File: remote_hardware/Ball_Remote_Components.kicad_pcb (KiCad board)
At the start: 4 copper layers, 92.3 x 128.5 mm, 77 parts, among them J1 Eurorack_10_pin_power, J2 SWD_Header, J3 USB_B_Micro, J4 X_Out, J5 Y_Out, J6 Z_Out, U1 STM32WB35, U2 LD1117-3.3-4Tab, U3 TL074, U4 TL072, Y1 32MHz

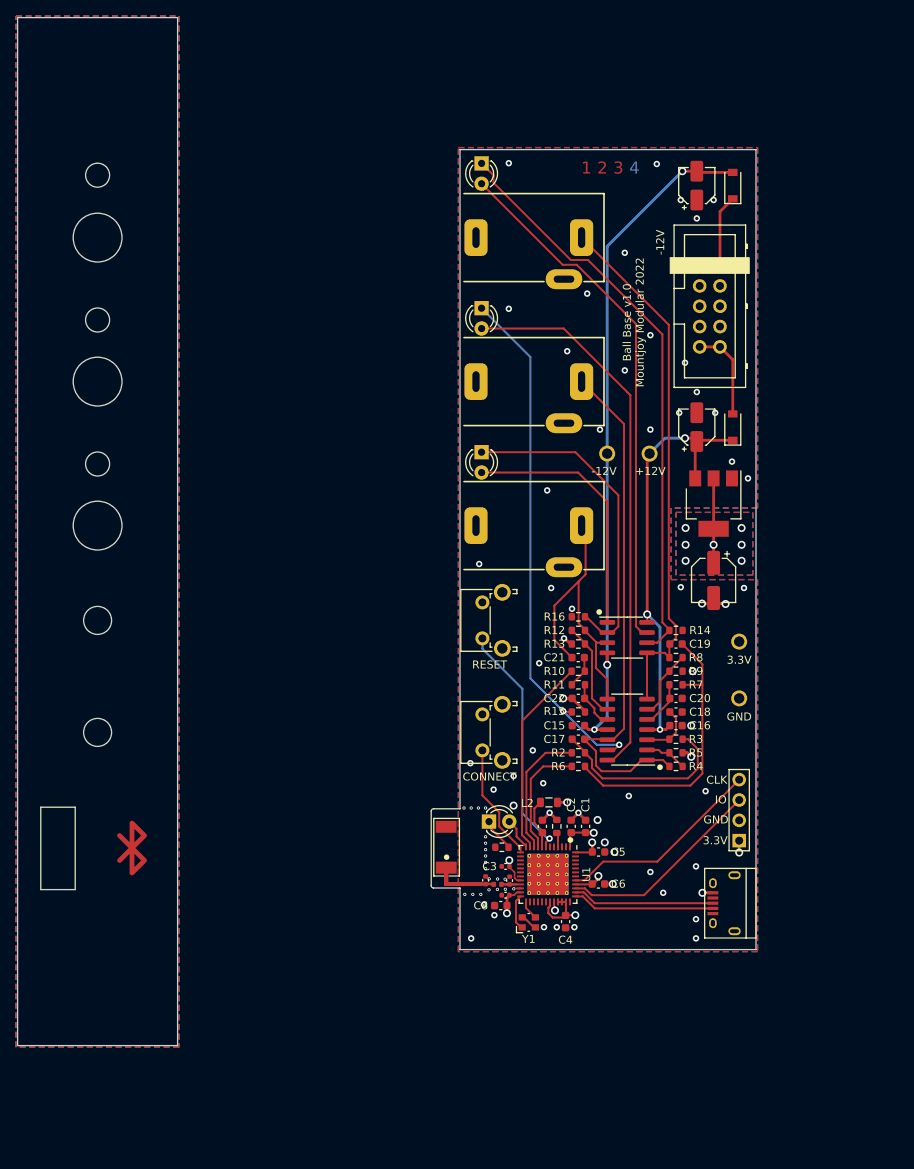
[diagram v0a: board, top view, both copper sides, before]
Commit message: Work on remote PCB
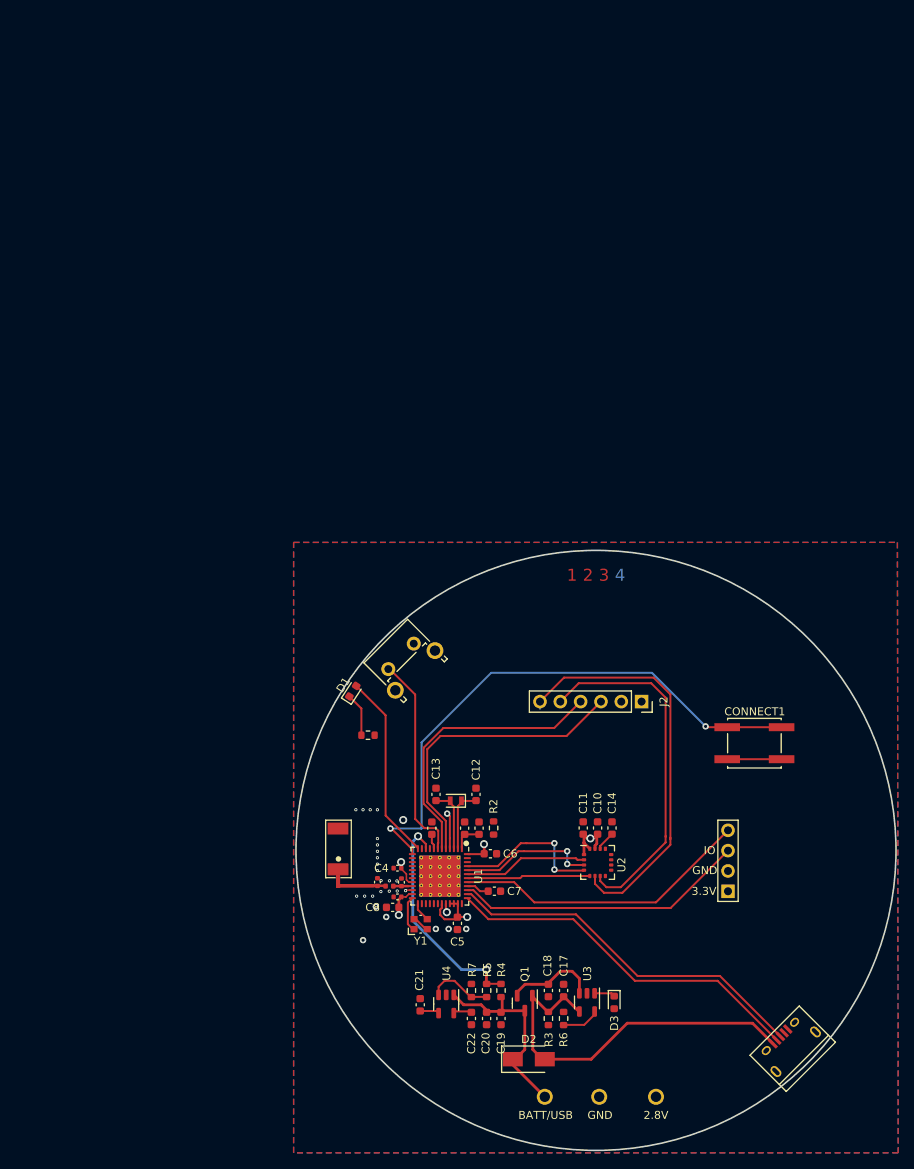
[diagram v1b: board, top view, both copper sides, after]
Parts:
- removed the C15 at (140.4, 128.0)
- removed the C16 at (152.6, 128.0)
- removed the D1 at (159.7, 90.7)
- removed D4: LED_X, LED_THT:LED_D3.0mm_FlatTop
- removed D5: LED_Y, LED_THT:LED_D3.0mm_FlatTop
- removed D6: LED_Z, LED_THT:LED_D3.0mm_FlatTop
- removed G***: LOGO, Custom_Footprints:bluetooth
- removed the J1 at (155.6, 70.5)
- removed J4: X_Out, Custom_Footprints:Jack_3.5mm_QingPu_WQP-PJ302M_Horizontal
- removed J5: Y_Out, Custom_Footprints:Jack_3.5mm_QingPu_WQP-PJ302M_Horizontal
- removed J6: Z_Out, Custom_Footprints:Jack_3.5mm_QingPu_WQP-PJ302M_Horizontal
- removed L2: L, Inductor_SMD:L_0805_2012Metric
- removed R10, R11: 20k, Resistor_SMD:R_0603_1608Metric
- removed R12, R8: 5k1, Resistor_SMD:R_0603_1608Metric
- removed R13, R9: 10k, Resistor_SMD:R_0603_1608Metric
- removed R14, R15, R16: 1k, Resistor_SMD:R_0603_1608Metric
- removed the R2 at (140.4, 131.4)
- removed Ref** (x3): Thonkikonn_6.1mm, Custom_Footprints:MountingHole_6.1mm
- removed Ref** (x3): LED_Hole_3mm, Custom_Footprints:LED_Hole_3mm
- removed Ref** (x2): Oval_Mounting_Hole, Custom_Footprints:Oval_Mounting_Hole
- removed Ref** (x2): Push_Button_Hole, Custom_Footprints:Small_Pushbutton_Hole_3.5mm
- removed TP4: TestPoint, Custom_Footprints:1.3mm_Test_Point
- added C12: 16pF, Capacitor_SMD:C_0603_1608Metric, F.Cu at (127.6, 136.6)
- added C13: 16pF, Capacitor_SMD:C_0603_1608Metric, F.Cu at (122.6, 136.6)
- added D3: LED_CHG, LED_SMD:LED_0603_1608Metric, F.Cu at (144.9, 162.6)
- added J2: I2C_Gyro_Module, Connector_PinSocket_2.54mm:PinSocket_1x06_P2.54mm_Vertical, F.Cu at (148.3, 125.0)
- added Q1: SI2333DS, Package_TO_SOT_SMD:SOT-23, F.Cu at (133.7, 162.7)
- added Y2: 32.768MHz, Crystal:Crystal_SMD_2012-2Pin_2.0x1.2mm, F.Cu at (125.1, 137.4)
- C10: value 22uF -> 100nF; footprint Capacitor_SMD:CP_Elec_4x5.4 -> Capacitor_SMD:C_0603_1608Metric
- C11: value 22uF -> 10uF; footprint Capacitor_SMD:CP_Elec_4x5.4 -> Capacitor_SMD:C_0603_1608Metric
- C14: value 47uF -> 10nF; footprint Capacitor_SMD:CP_Elec_5x5.8 -> Capacitor_SMD:C_0603_1608Metric
- C17: value 22nF -> 4.7uF
- C18: value 33nF -> 4.7uF
- C19: value 22nF -> 1uF
- C20, C22: value 33nF -> 1uF
- C21: value 22nF -> 10nF
- CONNECT1: footprint Button_Switch_THT:SW_Tactile_SPST_Angled_PTS645Vx58-2LFS -> Button_Switch_SMD:SW_SPST_EVQQ2
- D1: renamed from D3; value LED_BLUE -> LED_CONNECT; footprint LED_THT:LED_D3.0mm_FlatTop -> LED_SMD:LED_0603_1608Metric
- D2: value 1N5819 -> PMEG3010ER; footprint Diode_SMD:D_SOD-123 -> Diode_SMD:D_SMA
- R3: value 20k -> 1k
- R4: value 5k1 -> 27k
- R5: value 10k -> 13k
- R6: value 20k -> 10k
- R7: value 20k -> 24k
- U2: value LD1117-3.3-4Tab -> L3GD20; footprint Package_TO_SOT_SMD:SOT-223-3_TabPin2 -> Package_LGA:LGA-16_4x4mm_P0.65mm_LayoutBorder4x4y
- U3: value TL074 -> MCP73831-2-OT; footprint Package_SO:SOIC-14_3.9x8.7mm_P1.27mm -> Package_TO_SOT_SMD:SOT-23-5
- U4: value TL072 -> LD3985M28R_SOT23; footprint Package_SO:SOIC-8_3.9x4.9mm_P1.27mm -> Package_TO_SOT_SMD:SOT-23-5
- moved D2 112.1 mm to (134.2, 169.7), turned to 0 degrees
- moved C11 81.5 mm to (141.0, 140.8)
- moved TP3 81.5 mm to (136.2, 174.4), turned to -90 degrees
- moved TP2 57.8 mm to (150.1, 174.4), turned to 0 degrees
- moved TP1 52.8 mm to (143.0, 174.4), turned to 0 degrees
- moved C19 51.7 mm to (130.7, 164.6), turned to -90 degrees
- moved C10 51.6 mm to (142.8, 140.8)
- moved U4 51.1 mm to (123.9, 162.8), turned to -90 degrees
- moved FID1 50.9 mm to (142.6, 109.2)
- moved C21 47.7 mm to (120.6, 162.9), turned to 90 degrees
- moved U2 47.1 mm to (142.8, 145.1), turned to 0 degrees
- moved C20 46.5 mm to (128.9, 164.6), turned to -90 degrees
- moved R7 46.0 mm to (127.0, 161.1), turned to 90 degrees
- moved C22 42.2 mm to (127.0, 164.6), turned to -90 degrees
- moved R3 38.4 mm to (136.7, 164.6), turned to 90 degrees
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- renumbered C7 to C1, C12 to C15, C13 to C16, C1 to C2, C2 to C3, C3 to C4, C4 to C5, C5 to C6, C6 to C7, J3 to J1, J2 to J3, R17 to R1, R1 to R2
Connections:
- C1 pad 2: +3.3VA -> +2V8
- C10 pad 1: VCC -> +2V8
- C11 pad 1: GND -> +2V8
- C11 pad 2: VEE -> GND
- C14 pad 1: +3V3 -> Net-(C14-Pad1)
- C17 pad 1: /Y_Filtered -> /USB_VIN
- C17 pad 2: Net-(C17-Pad2) -> GND
- C18 pad 1: GND -> /BATT_+
- C18 pad 2: Net-(C18-Pad2) -> GND
- C19 pad 1: /X_Filtered -> VCC
- C19 pad 2: Net-(C19-Pad2) -> GND
- C2 pad 1: +3V3 -> +2V8
- C20 pad 1: GND -> VCC
- C20 pad 2: Net-(C20-Pad2) -> GND
- C21 pad 1: /Z_Filtered -> Net-(C21-Pad1)
- C21 pad 2: Net-(C21-Pad2) -> GND
- C22 pad 1: GND -> +2V8
- C22 pad 2: Net-(C22-Pad2) -> GND
- C3 pad 1: +3V3 -> +2V8
- C4 pad 1: +3V3 -> +2V8
- C5 pad 1: +3V3 -> +2V8
- C6 pad 1: +3V3 -> +2V8
- C7 pad 1: +3V3 -> +2V8
- C8 pad 1: +3V3 -> +2V8
- C9 pad 1: +3V3 -> +2V8
- D2 pad 1: -12V -> VCC
- D2 pad 2: VEE -> /USB_VIN
- J1 pad 1: unconnected-(J3-Pad1) -> /USB_VIN
- R3 pad 1: Net-(C17-Pad2) -> Net-(D3-Pad2)
- R3 pad 2: Net-(C18-Pad2) -> /USB_VIN
- R4 pad 1: Net-(R4-Pad1) -> VCC
- R4 pad 2: /Y_Filtered -> /Battery_Level
- R5 pad 1: GND -> /Battery_Level
- R5 pad 2: Net-(R4-Pad1) -> /LDO_Inhibit
- R6 pad 1: /X_PWM -> GND
- R6 pad 2: Net-(C19-Pad2) -> Net-(R6-Pad2)
- R7 pad 1: Net-(C19-Pad2) -> /LDO_Inhibit
- R7 pad 2: Net-(C20-Pad2) -> GND
- TP2 pad 1: +3V3 -> +2V8
- U1 pad 1: +3V3 -> +2V8
- U1 pad 10: /Y_PWM -> /Battery_Level
- U1 pad 11: /Z_PWM -> unconnected-(U1-Pad11)
- U1 pad 2: unconnected-(U1-Pad2) -> Net-(C12-Pad2)
- U1 pad 20: +3V3 -> +2V8
- U1 pad 23: +3V3 -> +2V8
- U1 pad 3: unconnected-(U1-Pad3) -> Net-(C13-Pad2)
- U1 pad 31: +3V3 -> +2V8
- U1 pad 33: +3V3 -> +2V8
- U1 pad 34: +3V3 -> +2V8
- U1 pad 35: +3V3 -> +2V8
- U1 pad 36: unconnected-(U1-Pad36) -> /LDO_Inhibit
- U1 pad 40: +3V3 -> +2V8
- U1 pad 42: unconnected-(U1-Pad42) -> /SPI_CS
- U1 pad 43: unconnected-(U1-Pad43) -> /SPI_CLK
- U1 pad 44: unconnected-(U1-Pad44) -> /SPI_MISO
- U1 pad 45: unconnected-(U1-Pad45) -> /SPI_MOSI
- U1 pad 48: +3V3 -> +2V8
- U1 pad 5: unconnected-(U1-Pad5) -> /I2C_CLK
- U1 pad 6: unconnected-(U1-Pad6) -> /12C_SDA
- U1 pad 8: +3.3VA -> +2V8
- U1 pad 9: /X_PWM -> unconnected-(U1-Pad9)
- U2 pad 1: GND -> +2V8
- U2 pad 2: +3V3 -> /SPI_CLK
- U2 pad 3: VCC -> /SPI_MISO
- U3 pad 1: /Y_Filtered -> /CHG_STAT
- U3 pad 2: Net-(R4-Pad1) -> GND
- U3 pad 3: Net-(C18-Pad2) -> /BATT_+
- U3 pad 4: VCC -> /USB_VIN
- U3 pad 5: Net-(C20-Pad2) -> Net-(R6-Pad2)
- U4 pad 1: Net-(D6-Pad2) -> VCC
- U4 pad 2: Net-(D6-Pad1) -> GND
- U4 pad 3: /Z_Filtered -> /LDO_Inhibit
- U4 pad 4: VEE -> Net-(C21-Pad1)
- U4 pad 5: /X_Filtered -> +2V8
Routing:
- net VEE: track 85.3 -> 0.00 mm, vias 3 -> 0
- net Net-(D4-Pad1): track 72.8 -> 0.00 mm
- net Net-(D5-Pad2): track 68.6 -> 0.00 mm
- net /X_Filtered: track 66.6 -> 0.00 mm
- net Net-(D5-Pad1): track 66.2 -> 0.00 mm, vias 2 -> 0
- net Net-(D4-Pad2): track 66.1 -> 0.00 mm
- net /Y_Filtered: track 65.4 -> 0.00 mm
- net /CONNECT: track 14.7 -> 70.5 mm, vias 0 -> 2
- net /G_RDY: track 0.00 -> 52.1 mm
- net /USB_VIN: track 0.00 -> 48.8 mm
- net /G_INT: track 0.00 -> 44.5 mm
- net Net-(D6-Pad1): track 41.0 -> 0.00 mm
- net +3V3: track 39.8 -> 0.00 mm, vias 15 -> 0
- net /I2C_CLK: track 0.00 -> 37.6 mm
- net +2V8: track 0.00 -> 37.4 mm, vias 0 -> 5
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- added copper zone on In2.Cu, net +2V8
- removed copper zone on B.Cu, net (none)
- removed copper zone on F.Cu, net (none)
- removed copper zone on B.Cu, net +3V3
- removed copper zone on F.Cu, net +3V3
- removed copper zone on In1.Cu, net +3V3
- removed copper zone on In2.Cu, net +3V3
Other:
- board size 92.3 x 128.5 mm -> 75 x 75 mm
- board text added: "2.8V"
- board text added: "BATT/USB"
- board text removed: "+12V"
- board text removed: "-12V"
- board text removed: "3.3V"
- board text removed: "Ball Base v1.0 Mountjoy Modular 2022"
- board text removed: "CONNECT"
- board text removed: "RESET"
